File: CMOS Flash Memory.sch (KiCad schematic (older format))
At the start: 2 parts, among them U5 28F010, U7 28F010

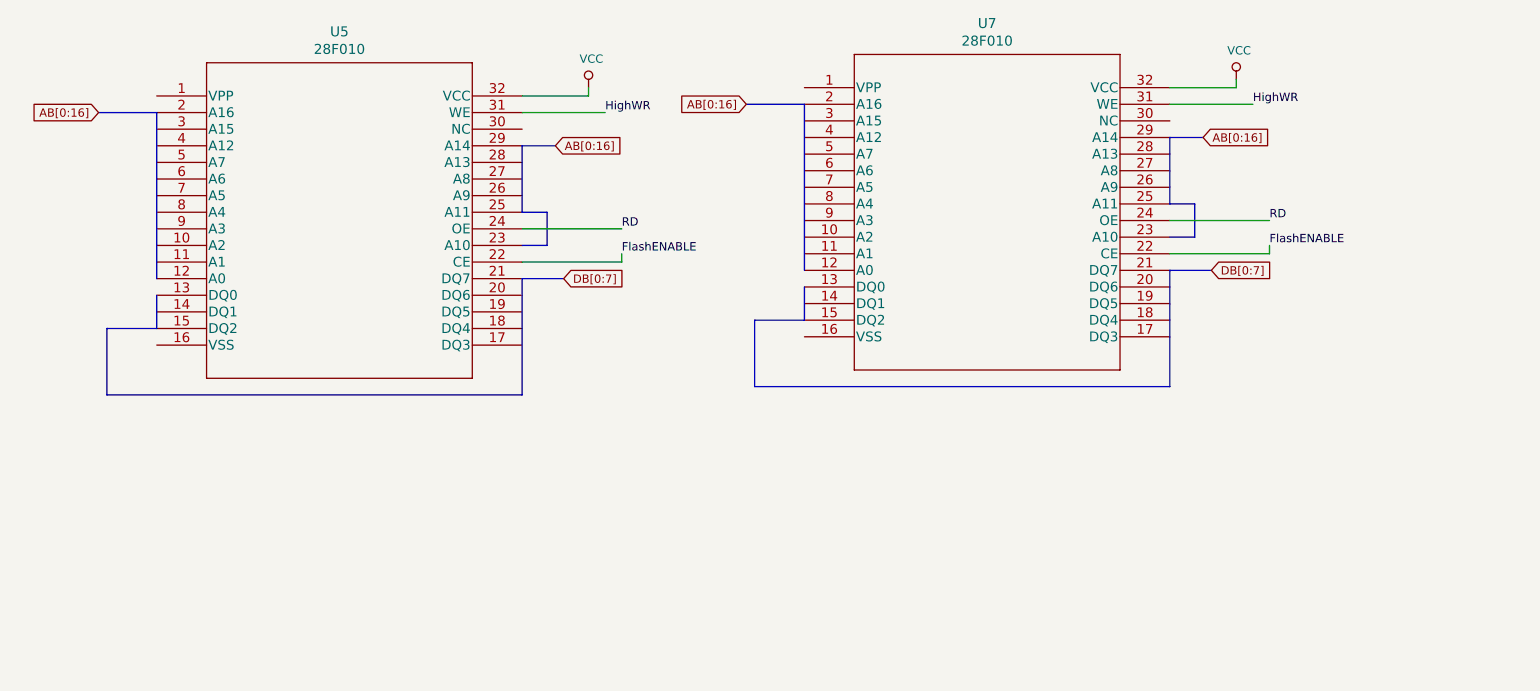
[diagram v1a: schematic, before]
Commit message: update
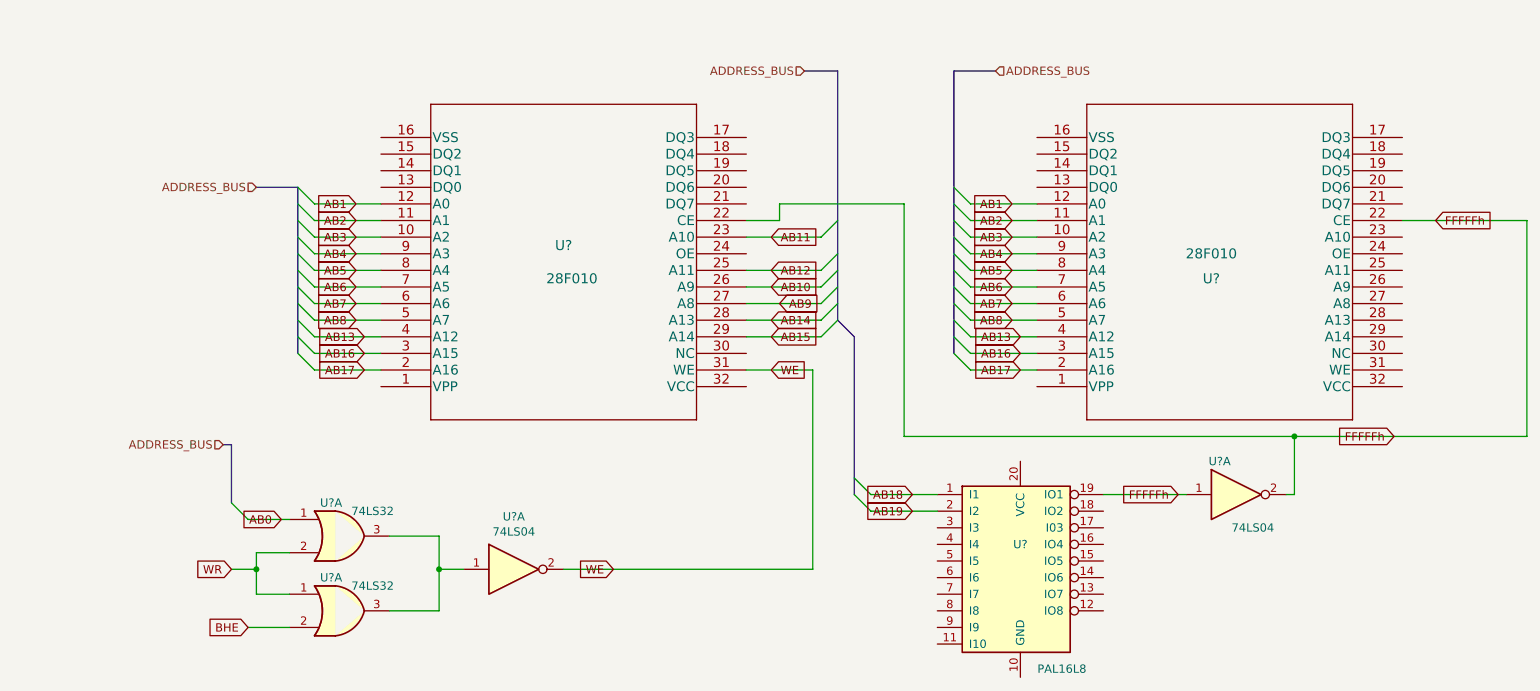
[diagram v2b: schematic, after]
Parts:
- removed U5, U7: 28F010, 28F010, symbol 28F010:28F010
- added U? (x2): 28F010, 28F010, symbol 28F010:28F010
- added U?: PAL16L8, symbol Logic_Programmable:PAL16L8
- added U? (x2): 74LS32, symbol 74xx:74LS32
- added U? (x2): 74LS04, symbol 74xx:74LS04
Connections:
- new net: U?.1, U?.3, U?.3
- new net AB0: U?.1
- new net AB1: U?.12 (A0), U?.12 (A0)
- new net AB10: U?.26 (A9)
- new net AB11: U?.23 (A10)
- new net AB12: U?.25 (A11)
- new net AB13: U?.4 (A12), U?.4 (A12)
- new net AB14: U?.28 (A13)
- new net AB15: U?.29 (A14)
- new net AB16: U?.3 (A15), U?.3 (A15)
- new net AB17: U?.2 (A16), U?.2 (A16)
- new net AB18: U?.1 (I1)
- new net AB19: U?.2 (I2)
- new net AB2: U?.11 (A1), U?.11 (A1)
- new net AB3: U?.10 (A2), U?.10 (A2)
- new net AB4: U?.9 (A3), U?.9 (A3)
- new net AB5: U?.8 (A4), U?.8 (A4)
- new net AB6: U?.7 (A5), U?.7 (A5)
- new net AB7: U?.6 (A6), U?.6 (A6)
- new net AB8: U?.5 (A7), U?.5 (A7)
- new net AB9: U?.27 (A8)
- new net BHE: U?.2
- new net FFFFFh: U?.1, U?.19 (IO1), U?.2, U?.22 (CE), U?.22 (CE)
- new net WE: U?.2, U?.31 (WE)
- new net WR: U?.1, U?.2
